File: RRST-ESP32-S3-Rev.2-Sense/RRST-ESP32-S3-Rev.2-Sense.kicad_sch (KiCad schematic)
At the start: 35 parts, among them J1 USB_C_Receptacle_USB2.0_16P, J4 Conn_01x05_Socket, J5 Conn_01x02_Socket, J6 Conn_01x02_Socket, SW1 SW_Push, SW2 SW_Push, U1 LD1117S33TR_SOT223, U2 ESP32-S3-WROOM-1, U3 MCP2561-E-SN

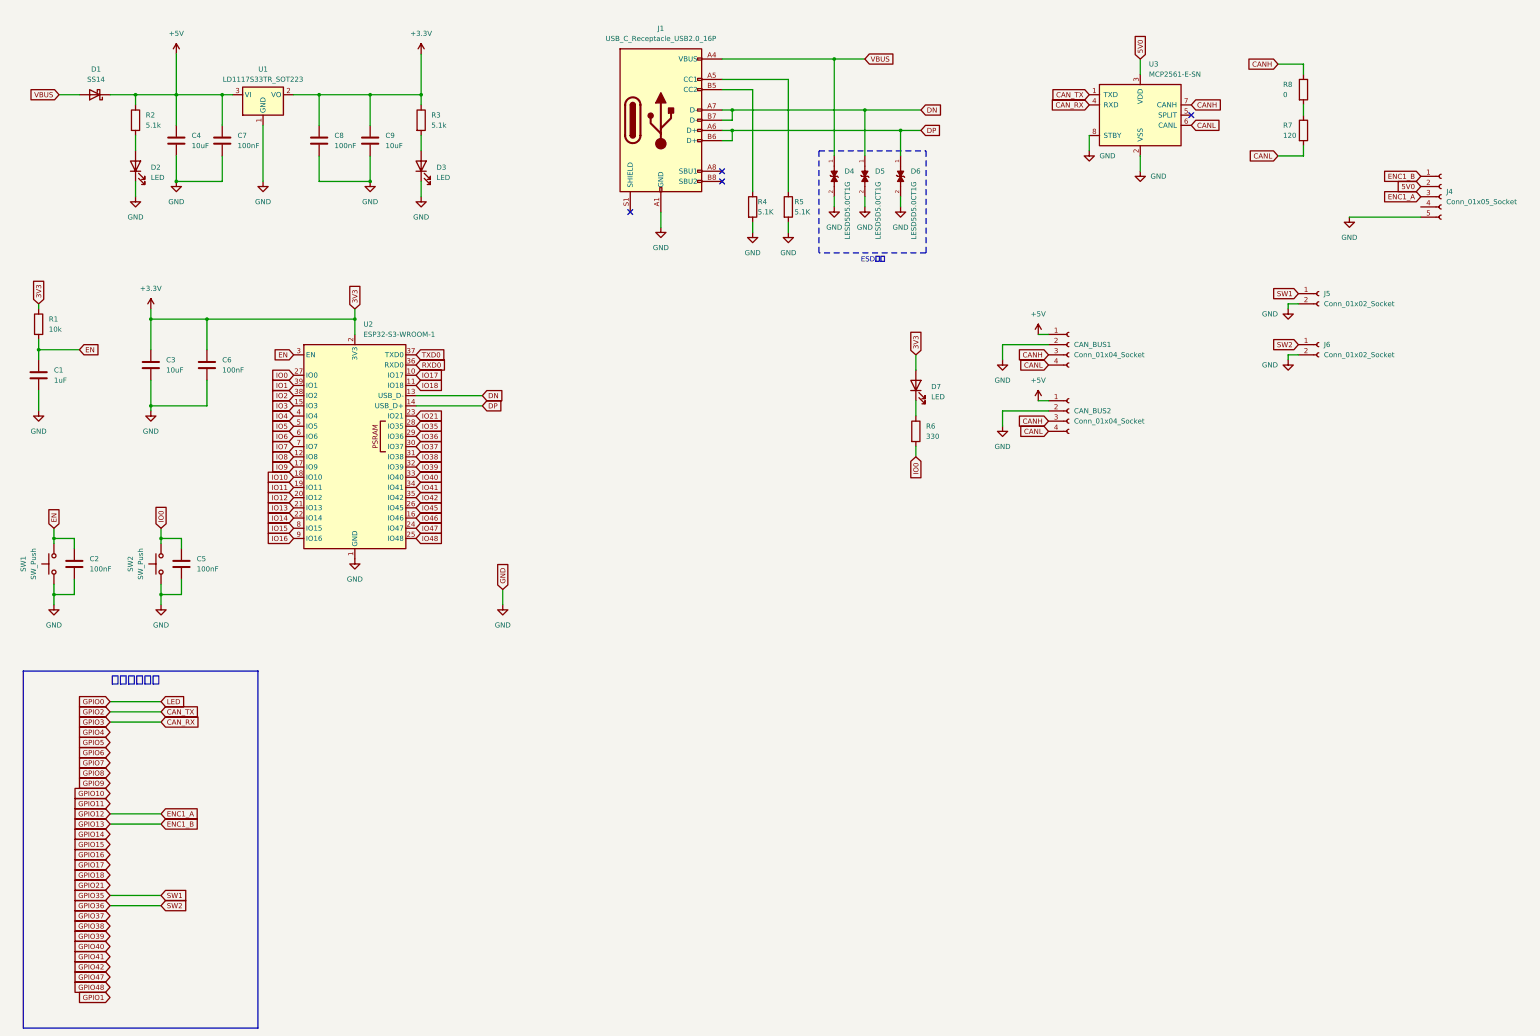
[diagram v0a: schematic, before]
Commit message: 自動配線前
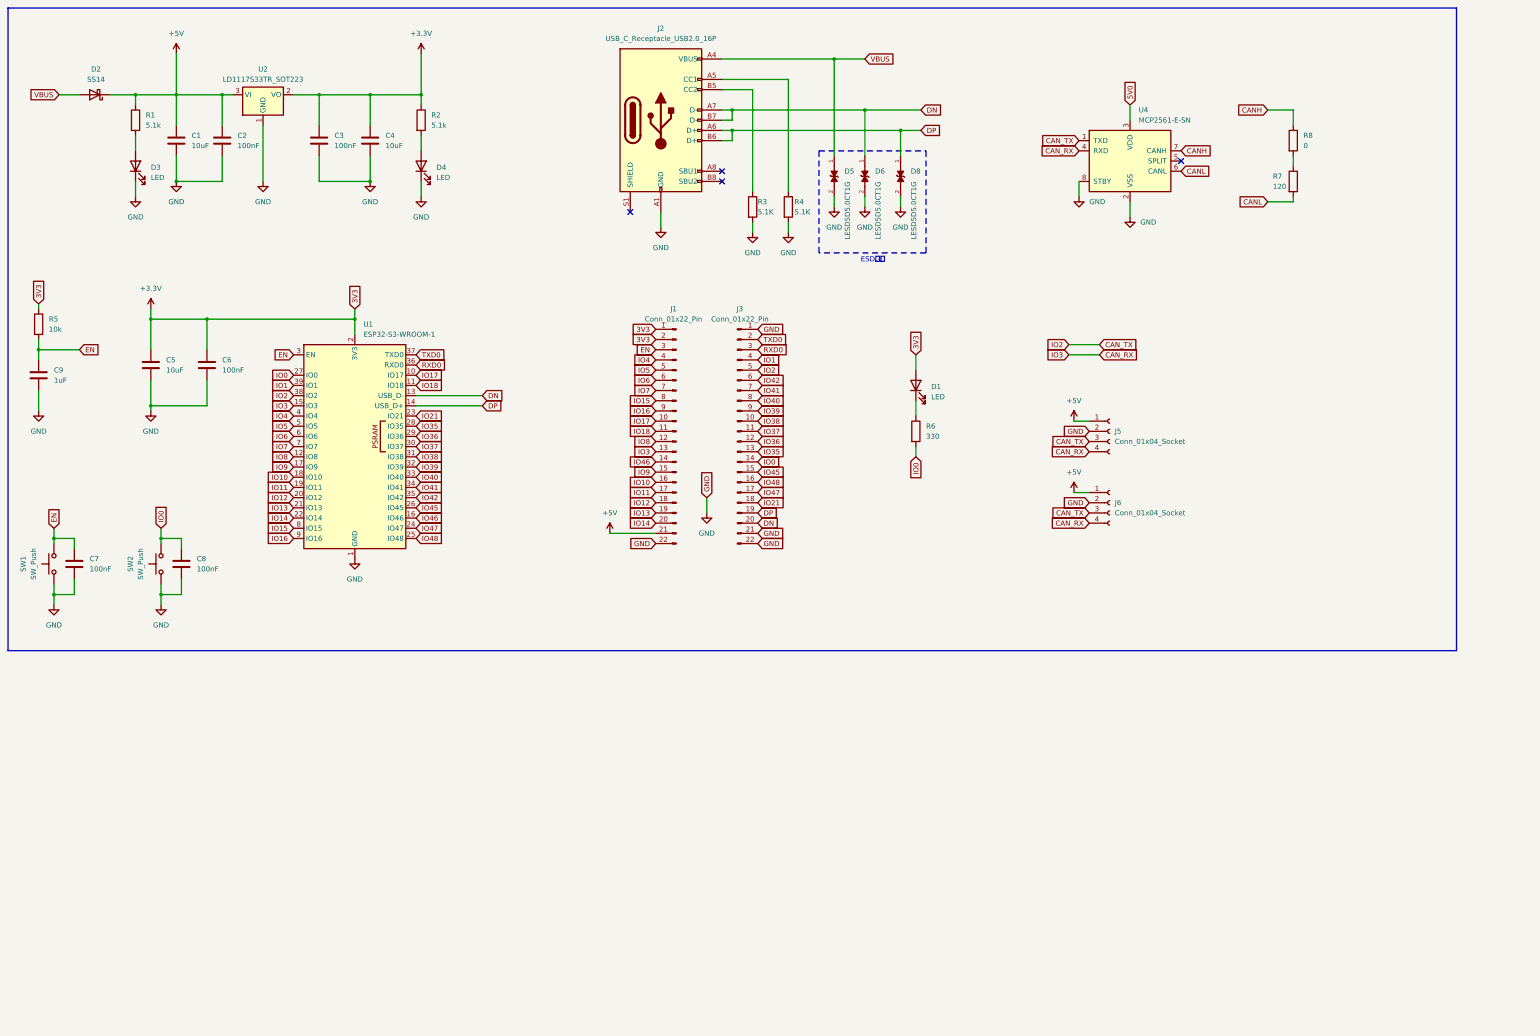
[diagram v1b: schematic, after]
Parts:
- removed CAN_BUS1, CAN_BUS2: Conn_01x04_Socket, Connector_JST:JST_GH_SM04B-GHS-TB_1x04-1MP_P1.25mm_Horizontal, symbol Connector:Conn_01x04_Socket
- removed J4: Conn_01x05_Socket, Connector_PinSocket_2.54mm:PinSocket_1x05_P2.54mm_Horizontal, symbol Connector:Conn_01x05_Socket
- removed J5, J6: Conn_01x02_Socket, Connector_JST:JST_PH_S2B-PH-K_1x02_P2.00mm_Horizontal, symbol Connector:Conn_01x02_Socket
- removed U3: MCP2561-E-SN, Package_SO:SOIC-8_3.9x4.9mm_P1.27mm, symbol Interface_CAN_LIN:MCP2561-E-SN
- added J1, J3: Conn_01x22_Pin, Connector_PinHeader_2.54mm:PinHeader_1x22_P2.54mm_Vertical, symbol Connector:Conn_01x22_Pin
- added J5, J6: Conn_01x04_Socket, Connector_JST:JST_XH_B4B-XH-A_1x04_P2.50mm_Vertical, symbol Connector:Conn_01x04_Socket
- added U4: MCP2561-E-SN, Package_SO:SOIC-8_3.9x4.9mm_P1.27mm, symbol Interface_CAN_LIN:MCP2561-E-SN
- R8: footprint Resistor_SMD:R_0603_1608Metric -> Resistor_SMD:R_0805_2012Metric
- renumbered C4 to C1, C7 to C2, C8 to C3, C9 to C4, C3 to C5, C2 to C7, C5 to C8, C1 to C9, D7 to D1, D1 to D2, D2 to D3, D3 to D4, D4 to D5, D5 to D6, D6 to D8, J1 to J2, R2 to R1, R3 to R2, R4 to R3, R5 to R4, R1 to R5, U2 to U1, U1 to U2
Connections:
- net IO2 is gone; now on net CAN_TX: U1.38 (IO2)
- net IO3 is gone; now on net CAN_RX: U1.15 (IO3)
- net +3.3V: now also J1.1 (Pin_1), J1.2 (Pin_2)
- net +5V: now also J1.21 (Pin_21), J5.1 (Pin_1), J6.1 (Pin_1)
- net 5V0: now also U4.3 (VDD)
- net CANH: now also U4.7 (CANH)
- net CANL: now also U4.6 (CANL)
- net CAN_RX: now also J1.13 (Pin_13), J5.4 (Pin_4), J6.4 (Pin_4), U4.4 (RXD)
- net CAN_TX: now also J3.5 (Pin_5), J5.3 (Pin_3), J6.3 (Pin_3), U4.1 (TXD)
- net DN: now also J3.20 (Pin_20)
- net DP: now also J3.19 (Pin_19)
- net EN: now also J1.3 (Pin_3)
- net GND: now also J1.22 (Pin_22), J3.1 (Pin_1), J3.21 (Pin_21), J3.22 (Pin_22), J5.2 (Pin_2), J6.2 (Pin_2), U4.2 (VSS), U4.8 (STBY)
- net IO0: now also J3.14 (Pin_14)
- net IO1: now also J3.4 (Pin_4)
- net IO10: now also J1.16 (Pin_16)
- net IO11: now also J1.17 (Pin_17)
- net IO12: now also J1.18 (Pin_18)
- net IO13: now also J1.19 (Pin_19)
- net IO14: now also J1.20 (Pin_20)
- net IO15: now also J1.8 (Pin_8)
- net IO16: now also J1.9 (Pin_9)
- net IO17: now also J1.10 (Pin_10)
- net IO18: now also J1.11 (Pin_11)
- net IO21: now also J3.18 (Pin_18)
- net IO35: now also J3.13 (Pin_13)
- net IO36: now also J3.12 (Pin_12)
- net IO37: now also J3.11 (Pin_11)
- net IO38: now also J3.10 (Pin_10)
- net IO39: now also J3.9 (Pin_9)
- net IO4: now also J1.4 (Pin_4)
- net IO40: now also J3.8 (Pin_8)
- net IO41: now also J3.7 (Pin_7)
- net IO42: now also J3.6 (Pin_6)
- net IO45: now also J3.15 (Pin_15)
- net IO46: now also J1.14 (Pin_14)
- net IO47: now also J3.17 (Pin_17)
- net IO48: now also J3.16 (Pin_16)
- net IO5: now also J1.5 (Pin_5)
- net IO6: now also J1.6 (Pin_6)
- net IO7: now also J1.7 (Pin_7)
- net IO8: now also J1.12 (Pin_12)
- net IO9: now also J1.15 (Pin_15)
- net RXD0: now also J3.3 (Pin_3)
- net TXD0: now also J3.2 (Pin_2)
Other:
- note removed: "ピン割り当て"
